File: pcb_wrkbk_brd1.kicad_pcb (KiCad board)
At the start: 2 copper layers, 35.3 x 39.1 mm, 41 parts, among them J1 ConnF_01x05, J2 USB_C_16Pin_C167321, J3 ConnM_01x03, U1 SA555DR, U2 LDO_3V3_2A_AIC1221-33GY3TR, U3 SN74ALVC14NSR, U4 LDO_5V_78D05AAL-TN3-R

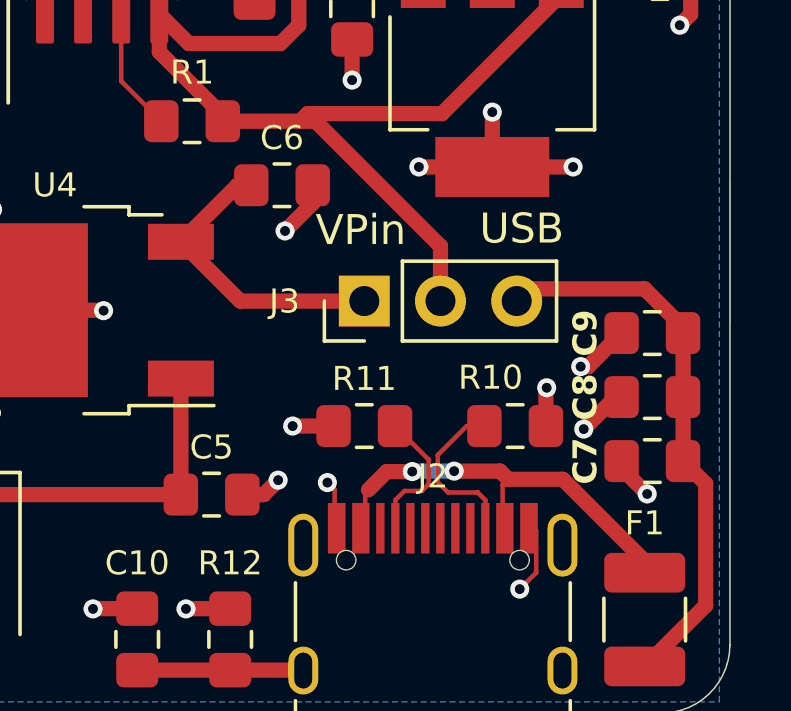
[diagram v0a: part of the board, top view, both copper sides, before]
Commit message: Updated with final files
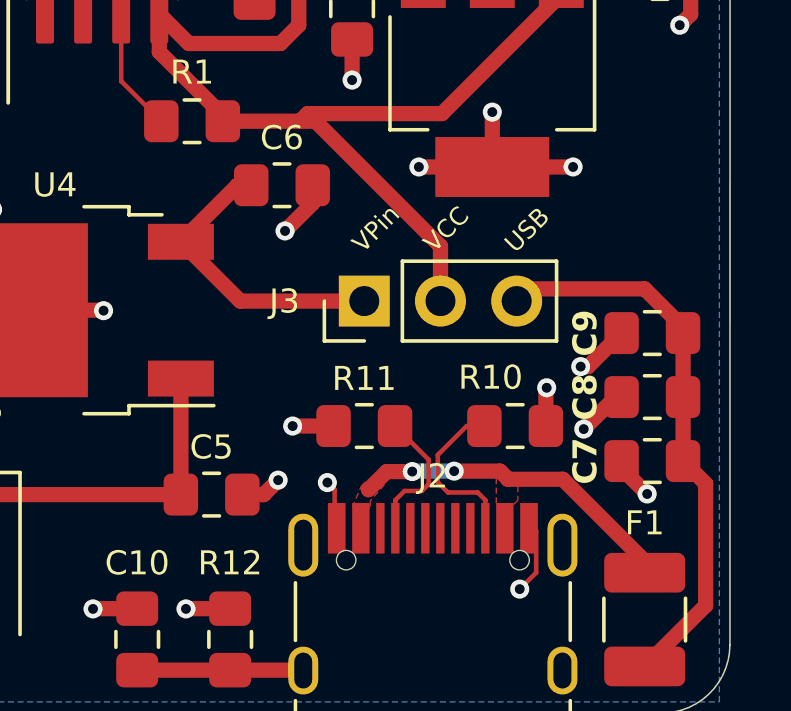
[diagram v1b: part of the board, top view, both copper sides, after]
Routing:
- net Net-(F1-Pad1): track 14.2 -> 11.3 mm
- added copper zone on F.Cu, net Net-(F1-Pad1)
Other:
- board text added: "VCC"
